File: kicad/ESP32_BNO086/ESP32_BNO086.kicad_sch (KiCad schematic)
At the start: 14 parts, among them IC1 BNO086, U1 XIAO-ESP32-C3/S3

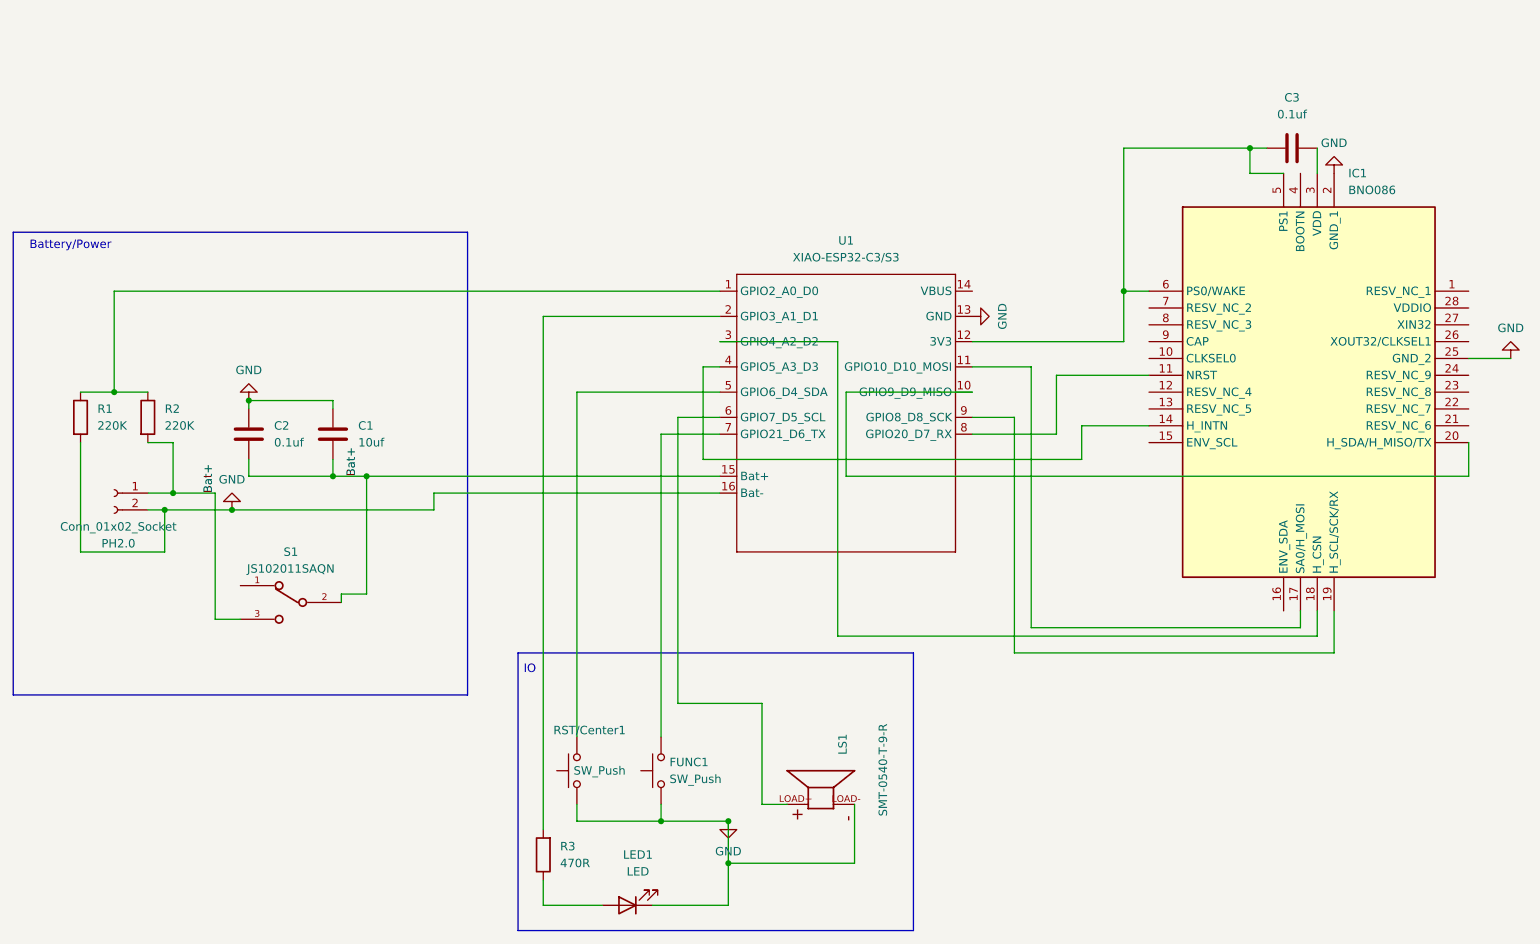
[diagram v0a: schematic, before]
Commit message: wiring changes
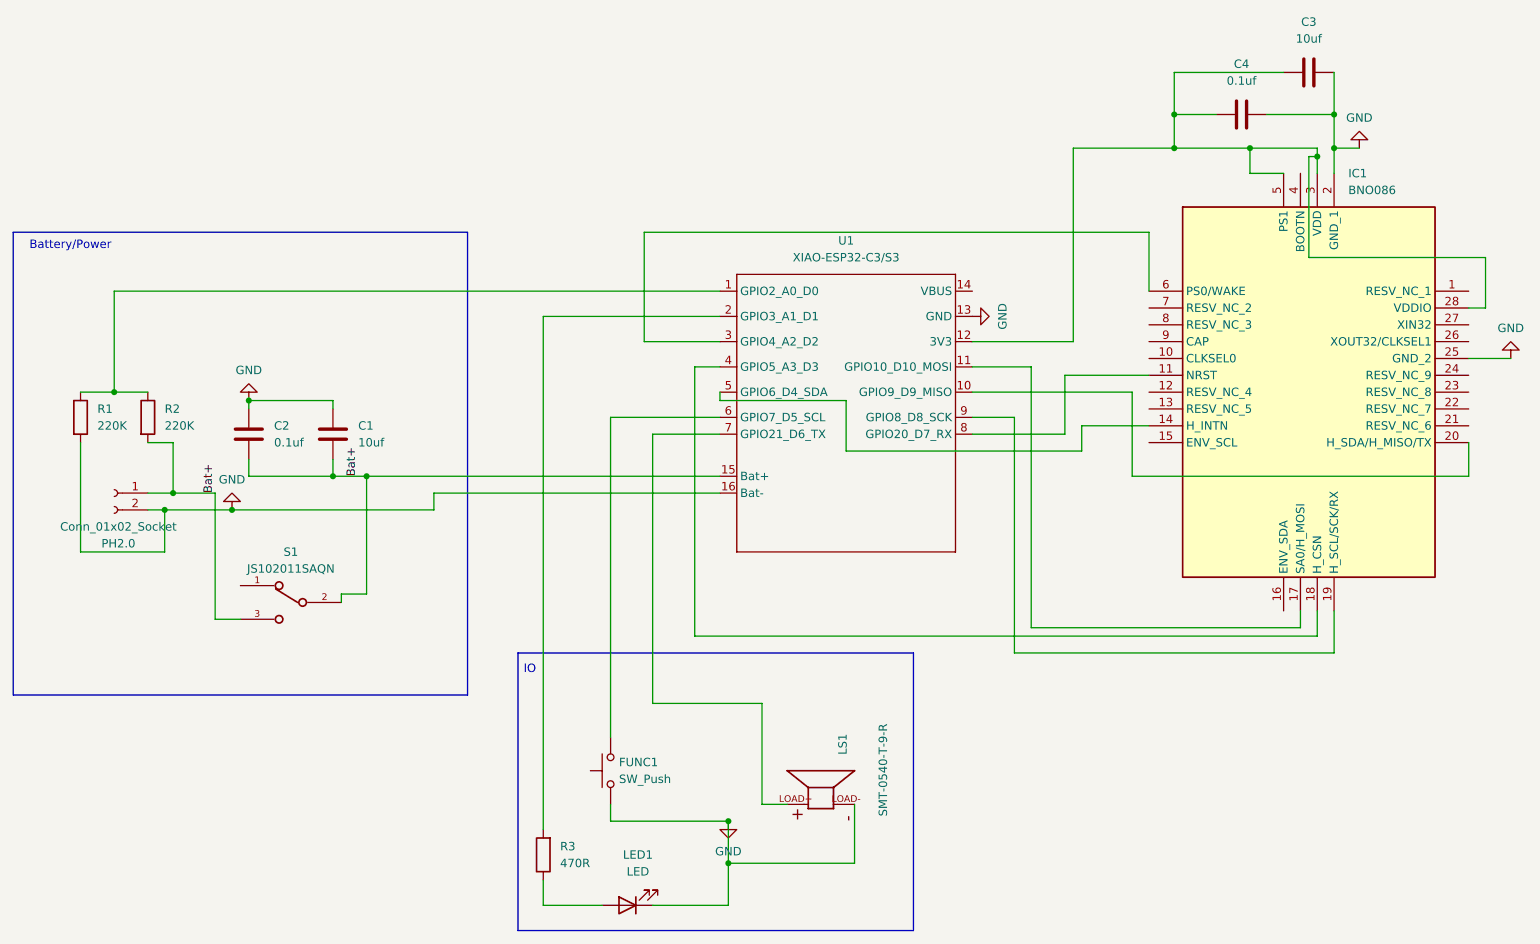
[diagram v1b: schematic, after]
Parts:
- removed RST/Center1: SW_Push, Button_Switch_SMD:SW_SPST_EVQP2_MiddlePushTravel_H2.5mm, symbol Switch:SW_Push
- added C4: 0.1uf, Capacitor_SMD:C_0402_1005Metric, symbol Device:C
- C3: value 0.1uf -> 10uf
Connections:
- net GND: now also C3.2, C4.2
- net at C3.1, IC1.5 (PS1), U1.12 (3V3): now also IC1.28 (VDDIO), IC1.3 (VDD), C4.1; no longer IC1.6 (PS0/WAKE)
- net at LS1.LOAD+: now also U1.7 (GPIO21_D6_TX); no longer U1.6 (GPIO7_D5_SCL)
- net at U1.5 (GPIO6_D4_SDA): now also IC1.14 (H_INTN)
- net at U1.3 (GPIO4_A2_D2): now also IC1.6 (PS0/WAKE); no longer IC1.18 (H_CSN)
- net at U1.4 (GPIO5_A3_D3): now also IC1.18 (H_CSN); no longer IC1.14 (H_INTN)
- net at FUNC1.2: now also U1.6 (GPIO7_D5_SCL); no longer U1.7 (GPIO21_D6_TX)
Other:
- moved on the sheet: C3, FUNC1
